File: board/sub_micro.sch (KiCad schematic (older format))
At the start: 5 parts, among them J301 USB_B, U301 STM32F072CBTx

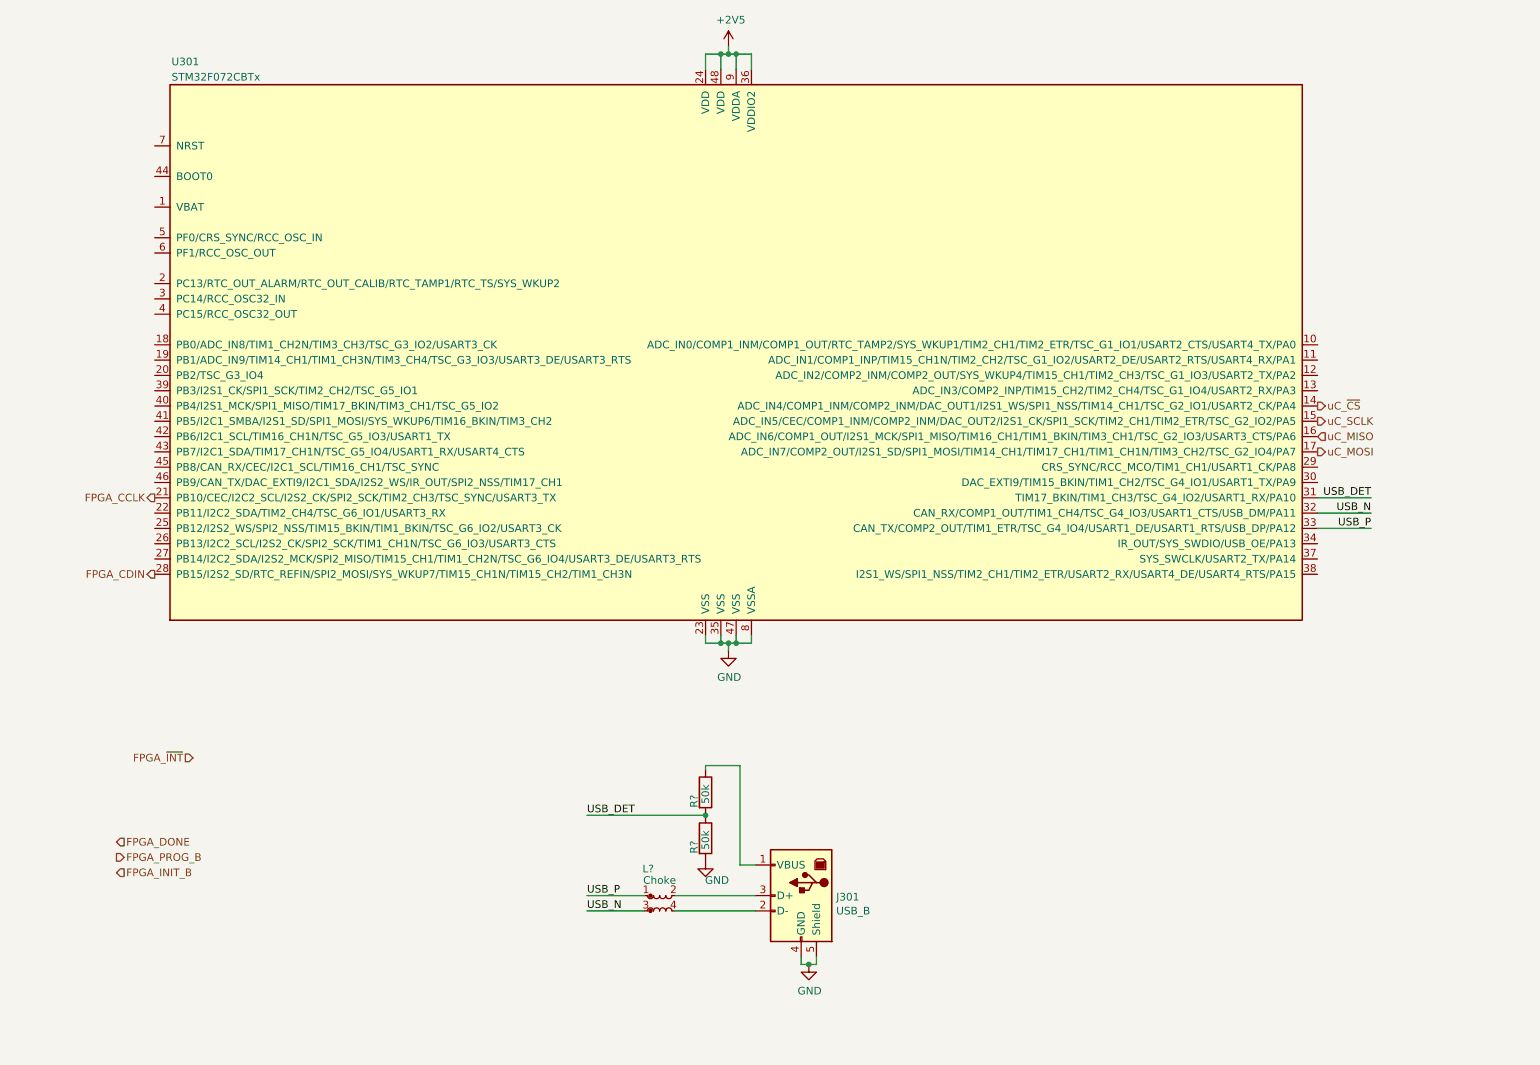
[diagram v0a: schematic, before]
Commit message: Schematics mostly complete
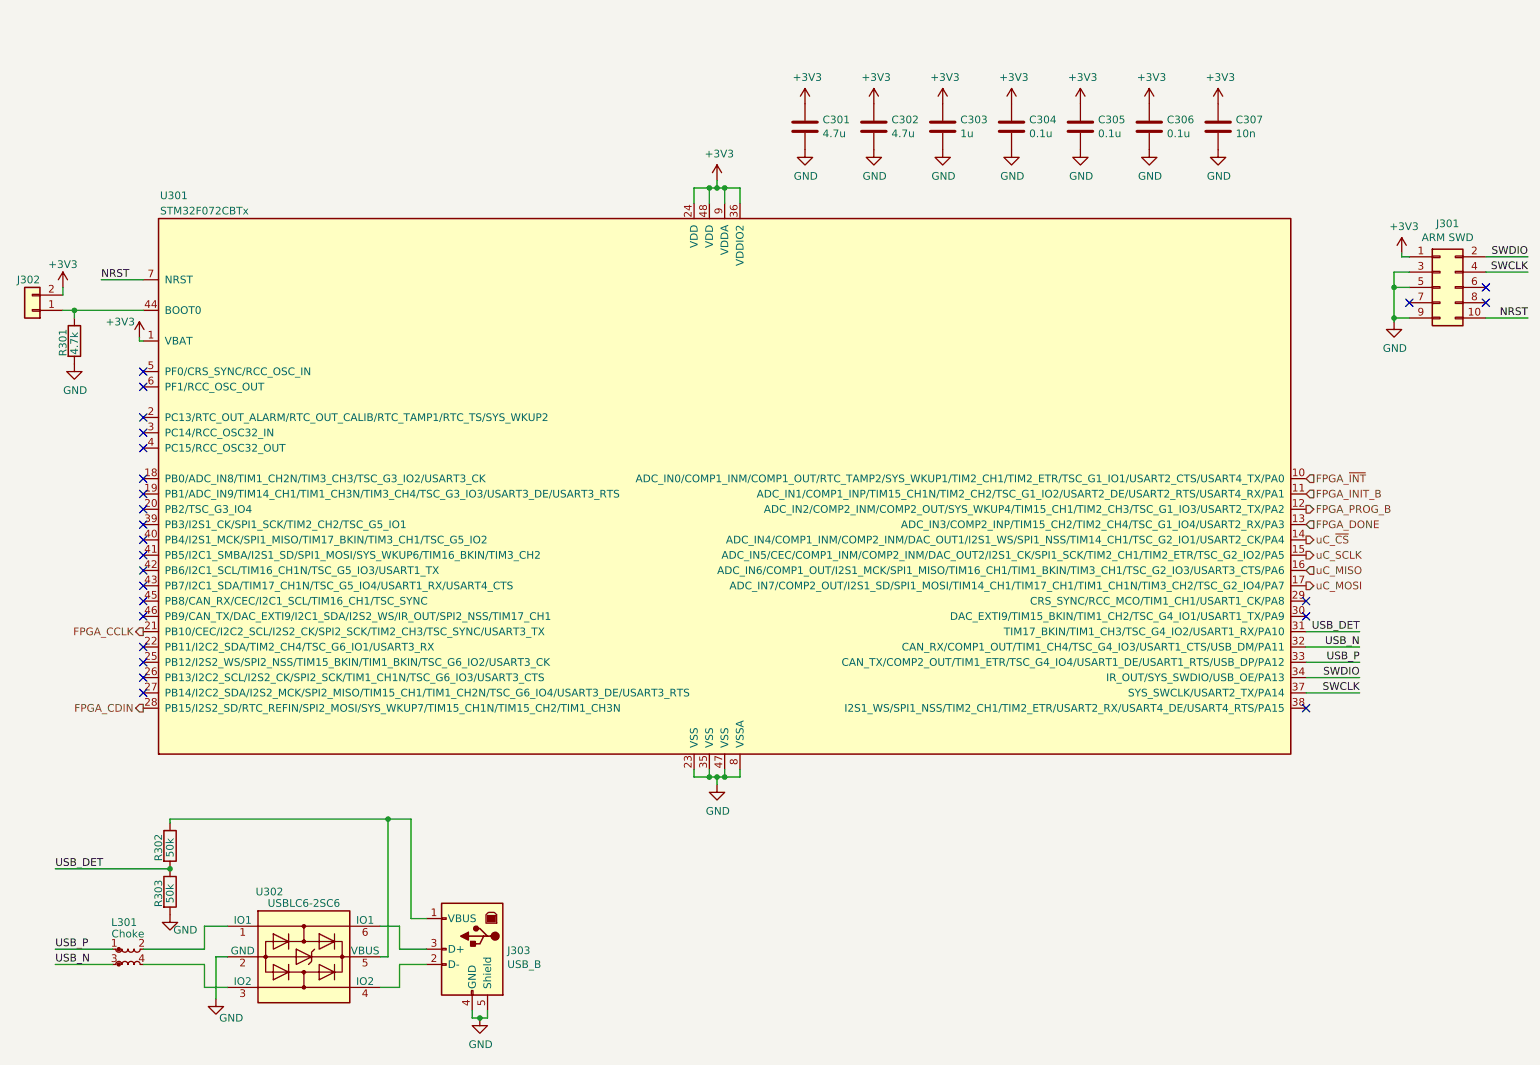
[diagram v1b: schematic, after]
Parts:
- added C301, C302: 4.7u, symbol Device:C
- added C303: 1u, symbol Device:C
- added C304, C305, C306: 0.1u, symbol Device:C
- added C307: 10n, symbol Device:C
- added J301: ARM SWD, symbol Connector_Generic:Conn_02x05_Odd_Even
- added J302: Conn_01x02, symbol Connector_Generic:Conn_01x02
- added R301: 4.7k, symbol Device:R
- added U302: USBLC6-2SC6, Package_TO_SOT_SMD:SOT-23-6, symbol quokka:USBLC6-2SC6
- gave numbers to parts that had none: 3
- renumbered J301 to J303
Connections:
- net +2V5 is gone; now on net +3V3: U301.24 (VDD), U301.36 (VDDIO2), U301.48 (VDD), U301.9 (VDDA)
- net FPGA_DONE: now also U301.13 (ADC_IN3/COMP2_INP/TIM15_CH2/TIM2_CH4/TSC_G1_IO4/USART2_RX/PA3)
- net FPGA_INIT_B: now also U301.11 (ADC_IN1/COMP1_INP/TIM15_CH1N/TIM2_CH2/TSC_G1_IO2/USART2_DE/USART2_RTS/USART4_RX/PA1)
- net FPGA_PROG_B: now also U301.12 (ADC_IN2/COMP2_INM/COMP2_OUT/SYS_WKUP4/TIM15_CH1/TIM2_CH3/TSC_G1_IO3/USART2_TX/PA2)
- net FPGA_~INT: now also U301.10 (ADC_IN0/COMP1_INM/COMP1_OUT/RTC_TAMP2/SYS_WKUP1/TIM2_CH1/TIM2_ETR/TSC_G1_IO1/USART2_CTS/USART4_TX/PA0)
- net GND: now also C301.2, C302.2, C303.2, C304.2, C305.2, C306.2, C307.2, J301.3 (Pin_3), J301.5 (Pin_5), J301.9 (Pin_9), R301.2, U302.2 (GND)
- net +3V3: now reaches U301.1 (VBAT)
- net +3V3: now also C301.1, C302.1, C303.1, C304.1, C305.1, C306.1, C307.1, J301.1 (Pin_1), J302.2 (Pin_2)
- net SWDIO: now reaches U301.34 (IR_OUT/SYS_SWDIO/USB_OE/PA13)
- net SWDIO: now also J301.2 (Pin_2)
- net SWCLK: now reaches U301.37 (SYS_SWCLK/USART2_TX/PA14)
- net SWCLK: now also J301.4 (Pin_4)
- net at U301.44 (BOOT0): now also J302.1 (Pin_1), R301.1
- net NRST: now reaches U301.7 (NRST)
- net NRST: now also J301.10 (Pin_10)
- net at J303.1 (VBUS), R302.1: now also U302.5 (VBUS)
- net at J303.2 (D-): now also U302.4 (IO2); no longer L301.4
- net at J303.3 (D+): now also U302.6 (IO1); no longer L301.2
- new net: L301.2, U302.1 (IO1)
- new net: L301.4, U302.3 (IO2)
- no-connect marks 0 -> 25
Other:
- moved on the sheet: J303, L301, R302, R303, U301
